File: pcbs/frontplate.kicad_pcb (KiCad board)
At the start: 2 copper layers, 133.3 x 91.7 mm, 5 parts

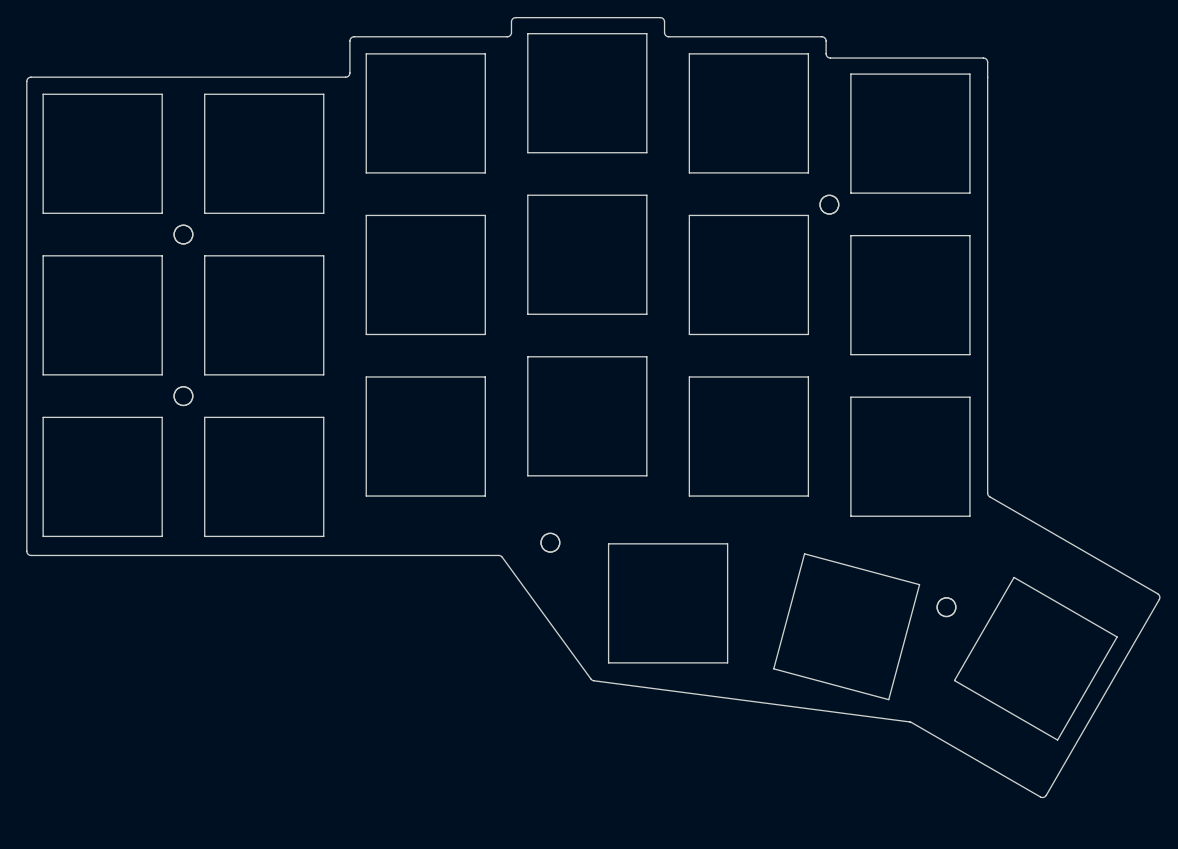
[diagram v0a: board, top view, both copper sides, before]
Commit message: ordered and working nicely.. need some adjustments
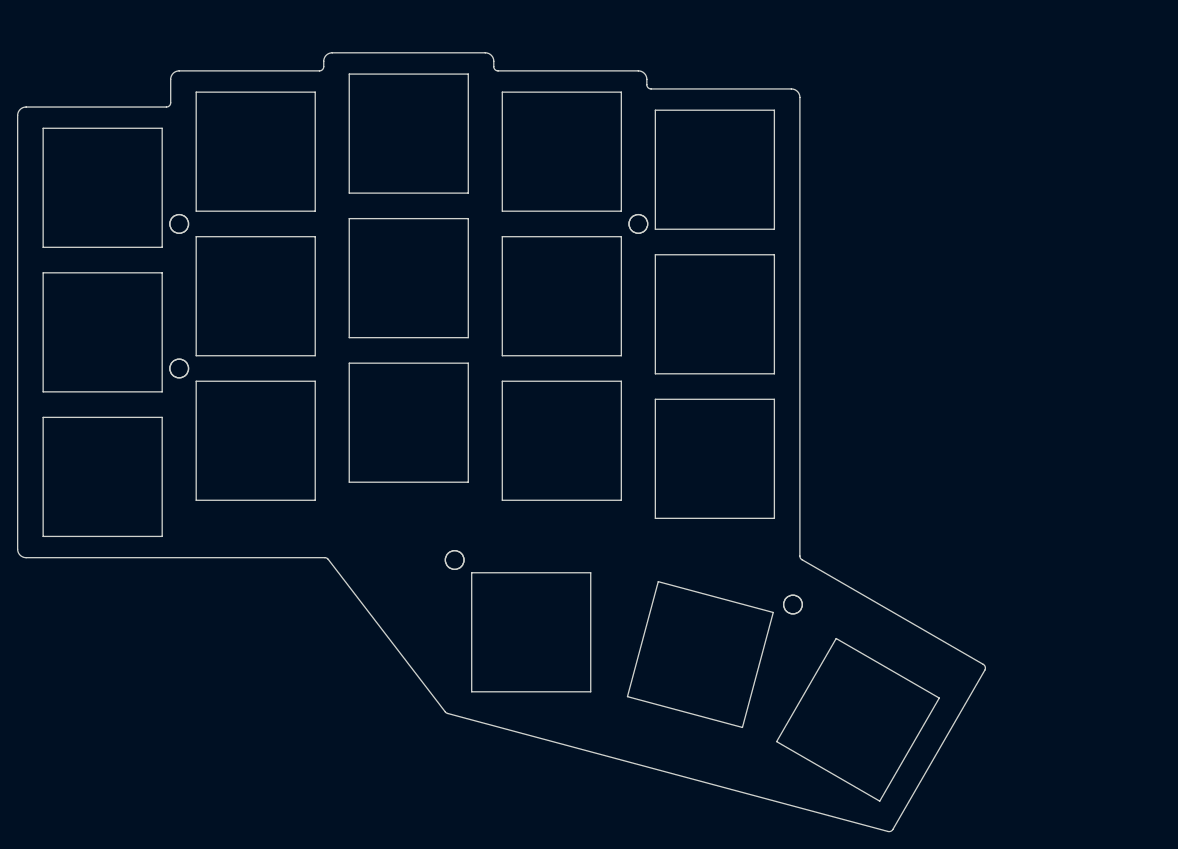
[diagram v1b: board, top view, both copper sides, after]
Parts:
- moved MH3 22.6 mm to (163.0, 70.2)
- moved MH5 18.1 mm to (181.2, 115.0), turned to -15 degrees
- moved MH4 11.4 mm to (141.4, 109.8)
- moved MH2 3.29 mm to (109.0, 87.2)
- moved MH1 1.35 mm to (109.0, 70.2)
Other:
- board size 133.3 x 91.7 mm -> 113.8 x 91.6 mm
